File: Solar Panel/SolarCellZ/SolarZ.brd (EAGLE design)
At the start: 91.1 x 91 mm, 34 parts, among them X1 BU-SMA-V

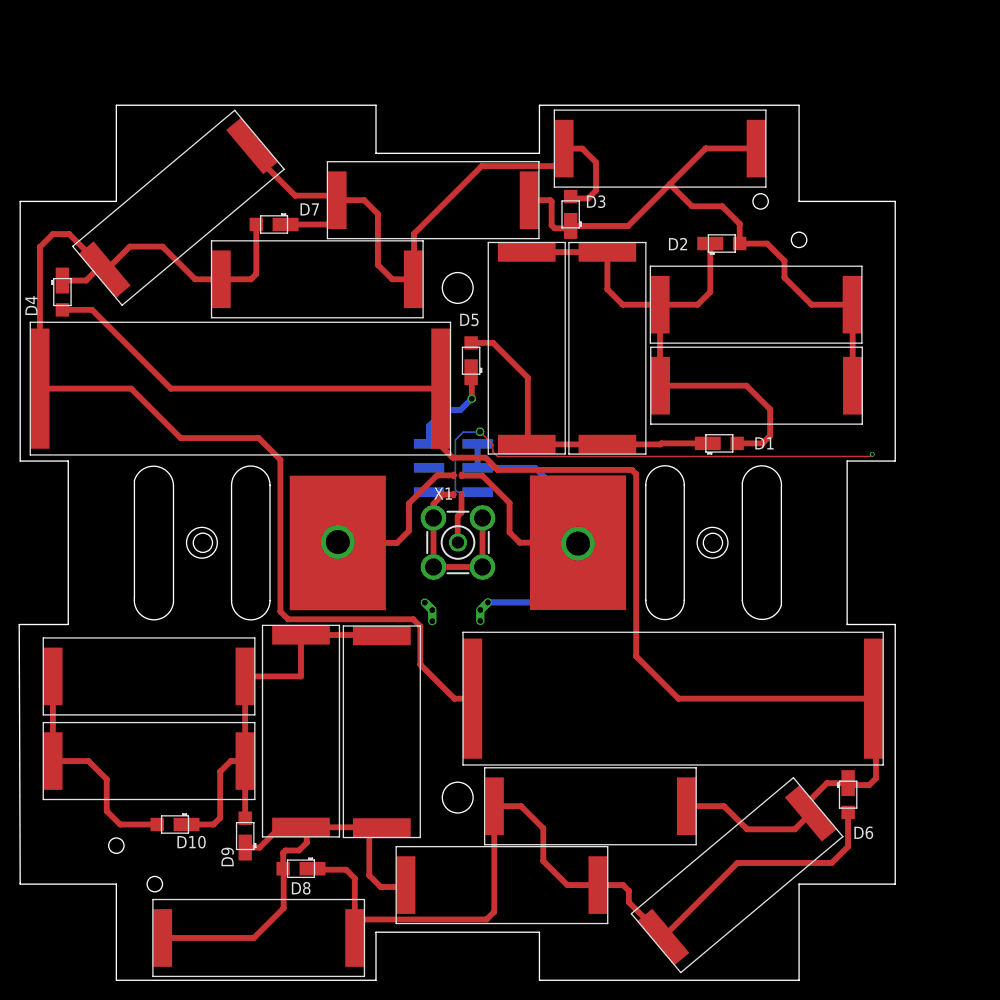
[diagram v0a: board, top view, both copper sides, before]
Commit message: Magnetorquers done
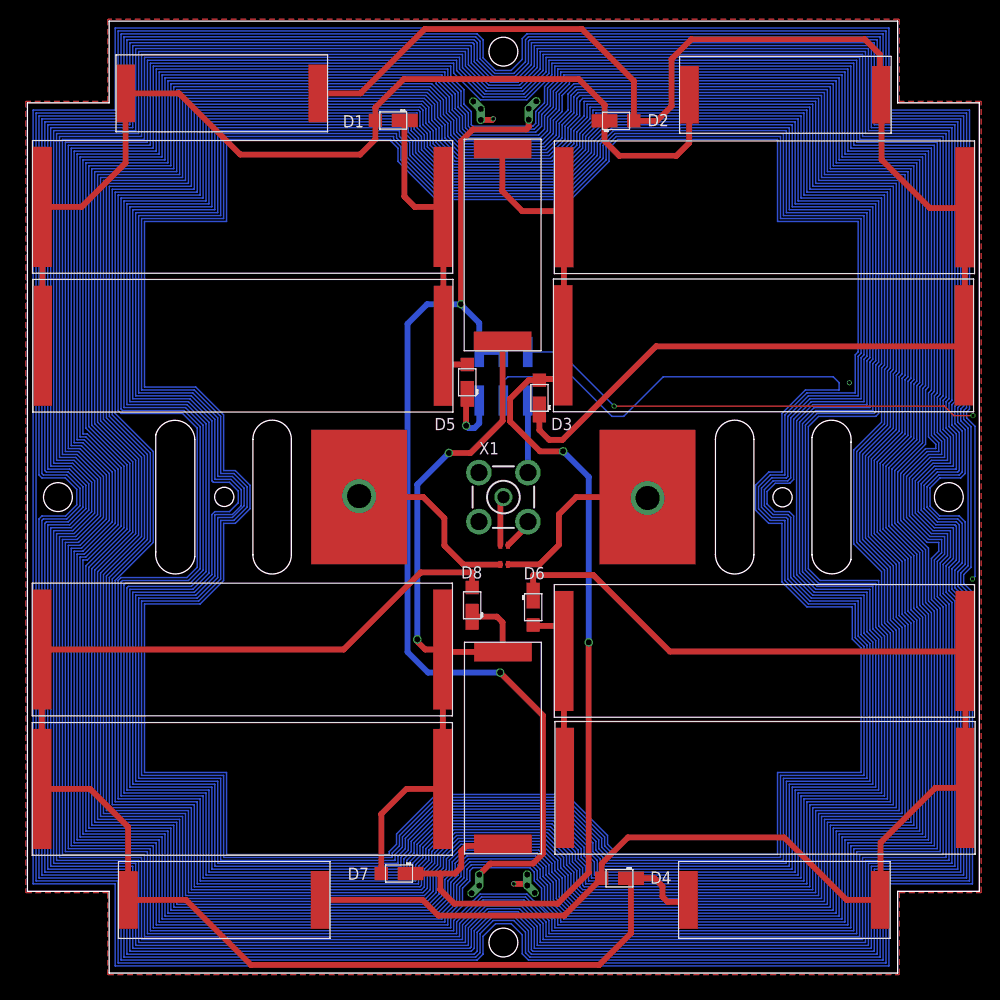
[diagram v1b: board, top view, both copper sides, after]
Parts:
- removed 15, 16, 17, 18: KXOB22-04X3F, Solar:KXOB22-04X3F
- removed D10, D9: SB_DIODE, Solar:SB_DIODE
- added F1: (no value), pandasat:BURN_WIRE
- 12, 14, 2, 3, 4, 5, 8, 9: value KXOB22-04X3F -> SLMD121H04L; device Solar:KXOB22-04X3F -> Solar:SLMD121H04L
- 6, 7: value SLMD121H04L -> KXOB22-04X3F; device Solar:SLMD121H04L -> Solar:KXOB22-04X3F
- moved D4 84.1 mm to (57.3, 5.61), turned to 180 degrees
- moved 6 72.3 mm to (85.5, 7.36)
- moved D7 68.7 mm to (34.4, 6.10)
- moved 7 62.3 mm to (27.2, 7.36)
- moved 1 59.8 mm to (27.0, 91.2)
- moved 3 55.9 mm to (-3.73, 68.5), turned to 0 degrees
- moved F2 52.4 mm to (42.9, 84.5)
- moved 2 50.6 mm to (-3.69, 54.1), turned to 0 degrees
- moved 10 50.0 mm to (41.2, 30.1), turned to 270 degrees
- moved D1 47.7 mm to (33.8, 84.4), turned to 180 degrees
- moved 12 43.6 mm to (-3.75, 22.5)
- moved D6 38.1 mm to (48.4, 33.8)
- moved 11 34.4 mm to (49.2, 60.5), turned to 90 degrees
- moved D8 32.7 mm to (42.0, 34.0), turned to 90 degrees
- moved 13 30.4 mm to (85.6, 91.1)
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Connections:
- removed net N$14: 12.P$1, 14.P$1, 15.P$2, 16.P$2, D8.POS, D9.NEG
- removed net N$18: 12.P$2, 14.P$2, 8.P$1, 9.P$1, D6.POS, D8.NEG
- removed net N$4: U$1.1, U$3.RF, U$3.RF_2
- new net N8: 12.P$1, 14.P$1, 6.P$2, 7.P$2, D4.NEG, D8.POS
- net GND: now also 8.P$1, 9.P$1, D6.POS, F1.2, F1.20, F1.200; no longer 17.P$1, 18.P$1, D10.POS
- net N$1: now also U$1.2, U$3.RF, U$3.RF_2; no longer 15.P$1, 16.P$1, 17.P$2, 18.P$2, D10.NEG, D9.POS
- net N$16: now also F1.1, F1.10, F1.100
- net N$3: now also U$1.1; no longer U$1.2
- net N$9: now also 12.P$2, 14.P$2, D8.NEG; no longer 6.P$2, 7.P$2, D4.NEG
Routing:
- net N$8: track 7354.4 -> 44659.3 mm, vias 2 -> 4
- net N8: track 0.00 -> 152.2 mm
- net N$10: track 64.5 -> 161.6 mm
- net N$18: track 91.2 -> 0.00 mm
- net N$16: track 32.2 -> 118.5 mm, vias 0 -> 2
- net N$6: track 56.6 -> 109.8 mm
- net N$12: track 68.1 -> 121.0 mm, vias 0 -> 2
- net N$14: track 50.9 -> 0.00 mm
- net N$9: track 121.9 -> 80.3 mm, vias 0 -> 2
- net N$1: track 44.9 -> 19.4 mm
- net N$4: track 16.7 -> 0.00 mm
- net GND: track 45.8 -> 39.3 mm, vias 0 -> 2
- net VSOLAR: track 10.3 -> 7.40 mm
- net N$3: track 16.8 -> 19.4 mm
- net N$7: track 33.3 -> 31.2 mm
- added copper zone on layer 1, net GND
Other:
- board size 91.1 x 91 mm -> 99 x 99 mm
